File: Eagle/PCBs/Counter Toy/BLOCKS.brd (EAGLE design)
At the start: 16 parts, among them Q1 2N7002

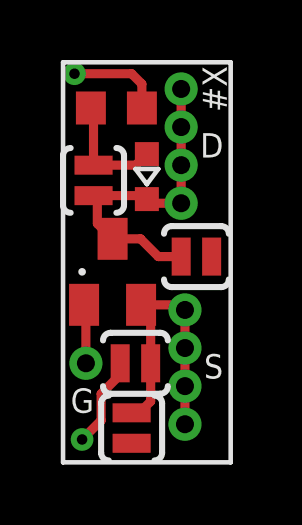
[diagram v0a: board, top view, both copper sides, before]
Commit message: Create LED output
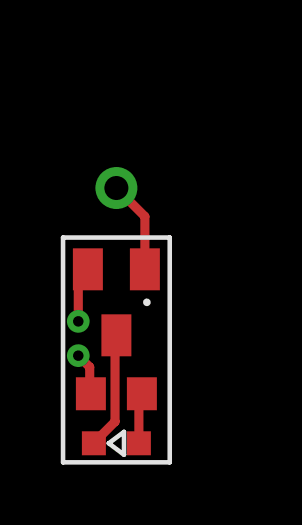
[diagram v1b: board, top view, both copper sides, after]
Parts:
- removed DRAINA1, DRAINB1, DRAINC1, DRAIND1, GATE1, SOURCEA1, SOURCEB1, SOURCEC1, SOURCED1: TPWIRE, ellajameson-core:TP_TH_WIRE
- removed JD1, JN1, JP1, JS1: SJ_NO, ellajameson-core:SJ_2S-NO
- added LED1: TPTHT, ellajameson-core:PROTOPAD-THT
- R1: value (none) -> 330
- moved R1 9.53 mm to (1.78, 2.29), turned to 180 degrees
- moved D1 8.95 mm to (1.78, 0.64), turned to 90 degrees
- moved Q1 1.02 mm to (1.78, 5.33), turned to 180 degrees
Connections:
- removed net N$6: D1.C, DRAINA1.TP, DRAINB1.TP, DRAINC1.TP, DRAIND1.TP, JD1.2, JP1.1, Q1.3
- removed net N$7: JN1.2, JS1.2, Q1.2, SOURCEA1.TP, SOURCEB1.TP, SOURCEC1.TP, SOURCED1.TP
- new net N$1: D1.C, Q1.3
- net GND: now also Q1.2; no longer JN1.1
- net N$5: no longer JP1.2
- net N$8: now also LED1.P1; no longer GATE1.TP
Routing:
- net N$6: track 11.0 -> 0.00 mm
- net N$7: track 9.49 -> 0.00 mm
- net N$1: track 0.00 -> 3.91 mm
- net N$5: track 3.87 -> 1.69 mm
- net VCC: track 3.19 -> 1.44 mm
- net GND: track 3.07 -> 1.87 mm
- net N$8: track 1.97 -> 3.10 mm
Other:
- board text removed: "#X"
- board text removed: "D"
- board text removed: "G"
- board text removed: "S"

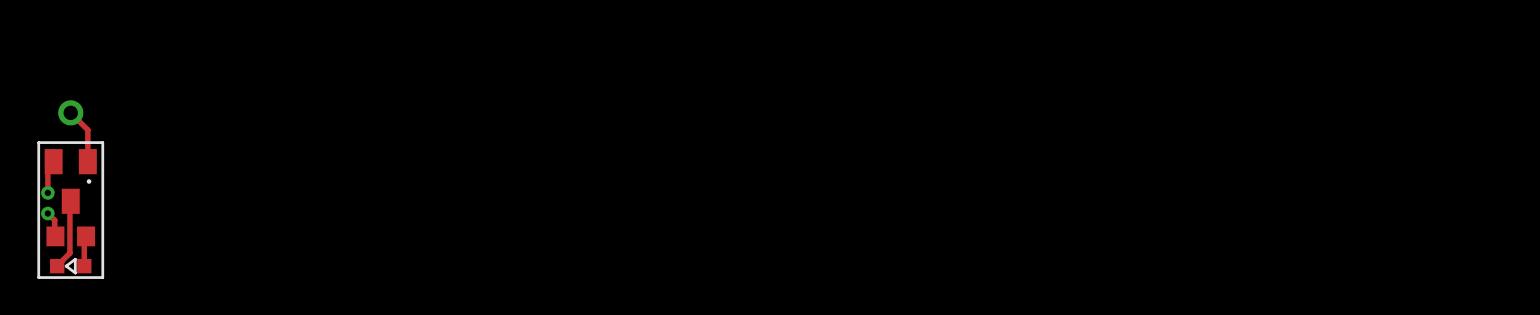
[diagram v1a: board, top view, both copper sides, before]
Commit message: Wow, 92 transistors and 8 LEDs
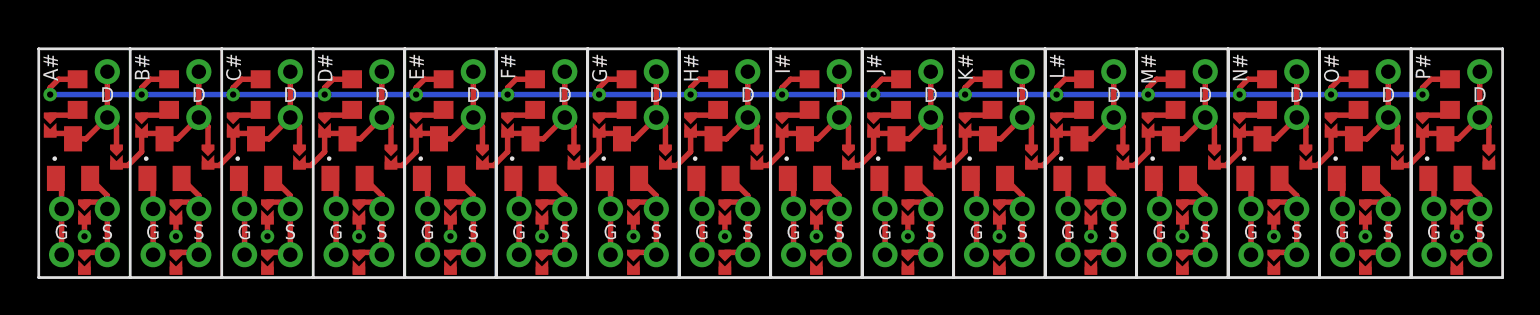
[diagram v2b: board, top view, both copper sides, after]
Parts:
- removed D1: (no value), ellajameson-core:CHIP-LED0603
- removed LED1: TPTHT, ellajameson-core:PROTOPAD-THT
- added DRAINA1, DRAINA10, DRAINA11, DRAINA12, DRAINA13, DRAINA14, DRAINA15, DRAINA16, DRAINA17, DRAINA18, DRAINA19, DRAINA20, DRAINA6, DRAINA7, DRAINA8, DRAINA9, DRAINB1, DRAINB10, DRAINB11, DRAINB12, DRAINB13, DRAINB14, DRAINB15, DRAINB16, DRAINB17, DRAINB18, DRAINB19, DRAINB20, DRAINB6, DRAINB7, DRAINB8, DRAINB9, GATEA1, GATEA10, GATEA11, GATEA12, GATEA13, GATEA14, GATEA15, GATEA16, GATEA17, GATEA18, GATEA19, GATEA20, GATEA6, GATEA7, GATEA8, GATEA9, GATEB1, GATEB10, GATEB11, GATEB12, GATEB13, GATEB14, GATEB15, GATEB16, GATEB17, GATEB18, GATEB19, GATEB20, GATEB6, GATEB7, GATEB8, GATEB9, SOURCEA1, SOURCEA10, SOURCEA11, SOURCEA12, SOURCEA13, SOURCEA14, SOURCEA15, SOURCEA16, SOURCEA17, SOURCEA18, SOURCEA19, SOURCEA20, SOURCEA6, SOURCEA7, SOURCEA8, SOURCEA9, SOURCEB1, SOURCEB10, SOURCEB11, SOURCEB12, SOURCEB13, SOURCEB14, SOURCEB15, SOURCEB16, SOURCEB17, SOURCEB18, SOURCEB19, SOURCEB20, SOURCEB6, SOURCEB7, SOURCEB8, SOURCEB9: TPTHT, ellajameson-core:PROTOPAD-THT-PAD
- added JD1, JD10, JD11, JD12, JD13, JD14, JD15, JD16, JD17, JD18, JD19, JD20, JD6, JD7, JD8, JD9, JN1, JN10, JN11, JN12, JN13, JN14, JN15, JN16, JN17, JN18, JN19, JN20, JN6, JN7, JN8, JN9, JP1, JP10, JP11, JP12, JP13, JP14, JP15, JP16, JP17, JP18, JP19, JP20, JP6, JP7, JP8, JP9, JS1, JS10, JS11, JS12, JS13, JS14, JS15, JS16, JS17, JS18, JS19, JS20, JS6, JS7, JS8, JS9: SJ_NO_THIN, ellajameson-core:SJ_2S-NO-THIN
- added Q10, Q11, Q12, Q13, Q14, Q15, Q16, Q17, Q18, Q19, Q20, Q6, Q7, Q8, Q9: 2N7002, ellajameson-core:SOT23
- added R10, R11, R12, R13, R14, R15, R16, R17, R18, R19, R20, R6, R7, R8, R9: 10k, ellajameson-core:R0603
- R1: value 330 -> 10k
- moved R1 22.1 mm to (22.5, 10.2), turned to 90 degrees
- moved Q1 20.5 mm to (22.2, 6.60), turned to 0 degrees
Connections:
- removed net N$8: LED1.P1, Q1.1
- new net N$2: JN9.2, JS9.2, Q1.2, SOURCEA9.P1, SOURCEB9.P1
- new net N$21: JN1.2, JS1.2, Q6.2, SOURCEA1.P1, SOURCEB1.P1
- new net N$22: DRAINA1.P1, DRAINB1.P1, JD1.2, JP1.1, Q6.3
- new net N$23: GATEA1.P1, GATEB1.P1, Q6.1
- new net N$24: JP6.2, R7.1
- new net N$25: JN6.2, JS6.2, Q7.2, SOURCEA6.P1, SOURCEB6.P1
- new net N$26: DRAINA6.P1, DRAINB6.P1, JD1.1, JD6.2, JP6.1, Q7.3
- new net N$27: GATEA6.P1, GATEB6.P1, Q7.1
- new net N$28: JP7.2, R8.1
- new net N$29: JN7.2, JS7.2, Q8.2, SOURCEA7.P1, SOURCEB7.P1
- new net N$30: DRAINA7.P1, DRAINB7.P1, JD6.1, JD7.2, JP7.1, Q8.3
- new net N$31: GATEA7.P1, GATEB7.P1, Q8.1
- new net N$32: JP8.2, R9.1
- new net N$33: JN8.2, JS8.2, Q9.2, SOURCEA8.P1, SOURCEB8.P1
- new net N$34: DRAINA8.P1, DRAINB8.P1, JD7.1, JD8.2, JP8.1, Q9.3
- new net N$35: GATEA8.P1, GATEB8.P1, Q9.1
- new net N$36: GATEA9.P1, GATEB9.P1, Q1.1
- new net N$37: JP10.2, R10.1
- new net N$38: JN10.2, JS10.2, Q10.2, SOURCEA10.P1, SOURCEB10.P1
- new net N$39: DRAINA10.P1, DRAINB10.P1, JD10.2, JD9.1, JP10.1, Q10.3
- new net N$40: GATEA10.P1, GATEB10.P1, Q10.1
- new net N$41: JP11.2, R11.1
- new net N$42: JN11.2, JS11.2, Q11.2, SOURCEA11.P1, SOURCEB11.P1
- new net N$43: DRAINA11.P1, DRAINB11.P1, JD10.1, JD11.2, JP11.1, Q11.3
- new net N$44: GATEA11.P1, GATEB11.P1, Q11.1
- new net N$45: JP12.2, R12.1
- new net N$46: JN12.2, JS12.2, Q12.2, SOURCEA12.P1, SOURCEB12.P1
- new net N$47: DRAINA12.P1, DRAINB12.P1, JD11.1, JD12.2, JP12.1, Q12.3
- new net N$48: GATEA12.P1, GATEB12.P1, Q12.1
- new net N$49: JP13.2, R13.1
- new net N$50: JN13.2, JS13.2, Q13.2, SOURCEA13.P1, SOURCEB13.P1
- new net N$51: DRAINA13.P1, DRAINB13.P1, JD12.1, JD13.2, JP13.1, Q13.3
- new net N$52: GATEA13.P1, GATEB13.P1, Q13.1
- new net N$53: JP14.2, R14.1
- new net N$54: JN14.2, JS14.2, Q14.2, SOURCEA14.P1, SOURCEB14.P1
- new net N$55: DRAINA14.P1, DRAINB14.P1, JD13.1, JD14.2, JP14.1, Q14.3
- new net N$56: GATEA14.P1, GATEB14.P1, Q14.1
- new net N$57: JP15.2, R15.1
- new net N$58: JN15.2, JS15.2, Q15.2, SOURCEA15.P1, SOURCEB15.P1
- new net N$59: DRAINA15.P1, DRAINB15.P1, JD14.1, JD15.2, JP15.1, Q15.3
- new net N$60: GATEA15.P1, GATEB15.P1, Q15.1
- new net N$61: JP16.2, R16.1
- new net N$62: JN16.2, JS16.2, Q16.2, SOURCEA16.P1, SOURCEB16.P1
- new net N$63: DRAINA16.P1, DRAINB16.P1, JD15.1, JD16.2, JP16.1, Q16.3
- new net N$64: GATEA16.P1, GATEB16.P1, Q16.1
- new net N$65: JP17.2, R17.1
- new net N$66: JN17.2, JS17.2, Q17.2, SOURCEA17.P1, SOURCEB17.P1
- new net N$67: DRAINA17.P1, DRAINB17.P1, JD16.1, JD17.2, JP17.1, Q17.3
- new net N$68: GATEA17.P1, GATEB17.P1, Q17.1
- new net N$69: JP18.2, R18.1
- new net N$7: JP1.2, R6.1
- new net N$70: JN18.2, JS18.2, Q18.2, SOURCEA18.P1, SOURCEB18.P1
- new net N$71: DRAINA18.P1, DRAINB18.P1, JD17.1, JD18.2, JP18.1, Q18.3
- new net N$72: GATEA18.P1, GATEB18.P1, Q18.1
- new net N$73: JP19.2, R19.1
- new net N$74: JN19.2, JS19.2, Q19.2, SOURCEA19.P1, SOURCEB19.P1
- new net N$75: DRAINA19.P1, DRAINB19.P1, JD18.1, JD19.2, JP19.1, Q19.3
- new net N$76: GATEA19.P1, GATEB19.P1, Q19.1
- new net N$77: JP20.2, R20.1
- new net N$78: JN20.2, JS20.2, Q20.2, SOURCEA20.P1, SOURCEB20.P1
- new net N$79: DRAINA20.P1, DRAINB20.P1, JD19.1, JD20.2, JP20.1, Q20.3
- new net N$80: GATEA20.P1, GATEB20.P1, Q20.1
- net GND: now also JN1.1, JN10.1, JN11.1, JN12.1, JN13.1, JN14.1, JN15.1, JN16.1, JN17.1, JN18.1, JN19.1, JN20.1, JN6.1, JN7.1, JN8.1, JN9.1; no longer Q1.2
- net N$1: now also JP9.2, R1.1; no longer D1.C, Q1.3
- net N$5: now also DRAINA9.P1, DRAINB9.P1, JD8.1, JD9.2, JP9.1, Q1.3; no longer D1.A, R1.1
- net VCC: now also R10.2, R11.2, R12.2, R13.2, R14.2, R15.2, R16.2, R17.2, R18.2, R19.2, R20.2, R6.2, R7.2, R8.2, R9.2
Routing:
- net VCC: track 1.44 -> 109.8 mm, vias 1 -> 16
- net GND: track 1.87 -> 14.2 mm, vias 1 -> 16
- net N$59: track 0.00 -> 10.9 mm
- net N$43: track 0.00 -> 10.9 mm
- net N$67: track 0.00 -> 10.9 mm
- net N$55: track 0.00 -> 10.9 mm
- net N$34: track 0.00 -> 10.9 mm
- net N$30: track 0.00 -> 10.9 mm
- net N$26: track 0.00 -> 10.9 mm
- net N$79: track 0.00 -> 10.9 mm
- net N$71: track 0.00 -> 10.9 mm
- net N$63: track 0.00 -> 10.9 mm
- net N$51: track 0.00 -> 10.9 mm
- net N$39: track 0.00 -> 10.9 mm
- net N$75: track 0.00 -> 10.9 mm
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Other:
- board text added: "A#"
- board text added: "B#"
- board text added: "C#"
- board text added: "D"
- board text added: "D#"
- board text added: "E#"
- board text added: "F#"
- board text added: "G"
- board text added: "G#"
- board text added: "H#"
- board text added: "I#"
- board text added: "J#"
- board text added: "K#"
- board text added: "L#"
- board text added: "M#"
- board text added: "N#"
- board text added: "O#"
- board text added: "P#"
- board text added: "S"
